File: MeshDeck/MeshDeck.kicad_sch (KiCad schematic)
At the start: 18 parts, among them CN1 ATGM336H-6N-74, SW1 4*4*1.7, SW2 4*4*1.7, U1 ESP32-S3-WROOM-1(N16R8), U2 SX1262S8S+T-X1, U5 RN32768114

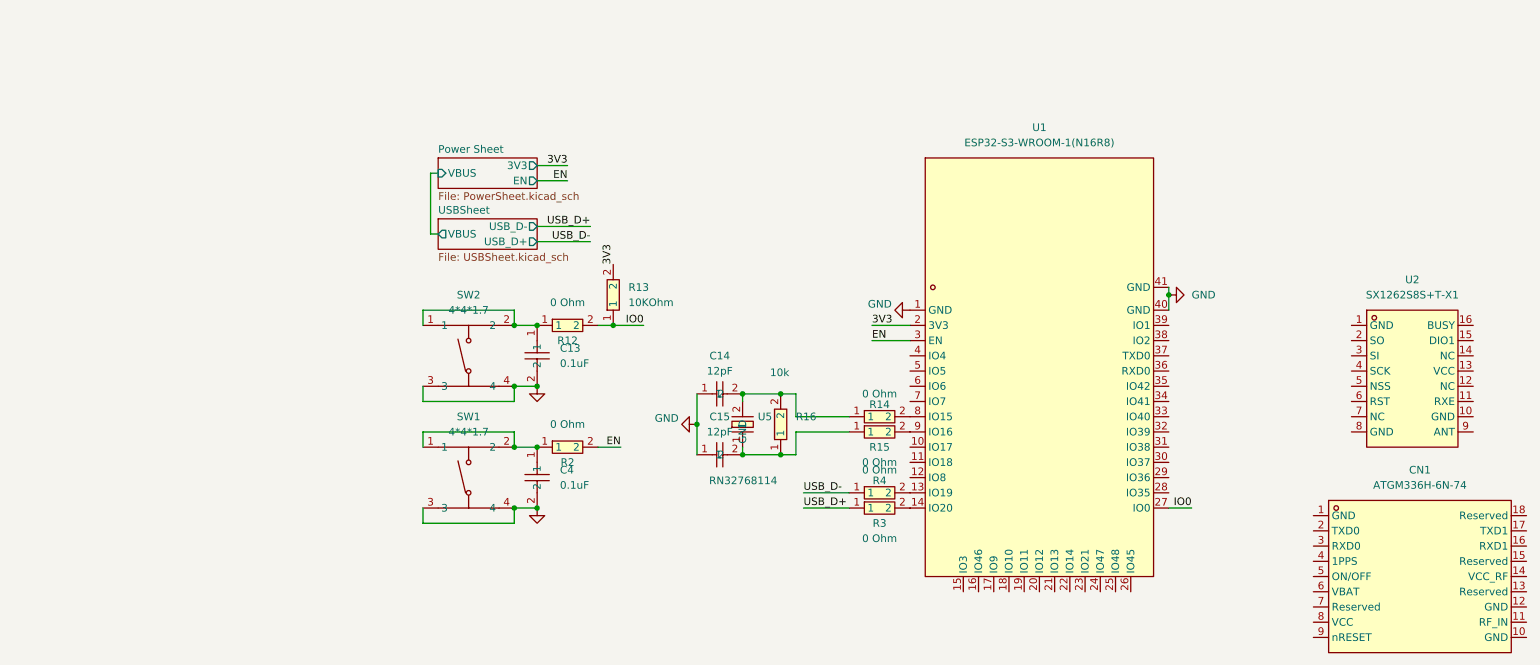
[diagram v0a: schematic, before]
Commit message: set up LoRa module and screen (wip)
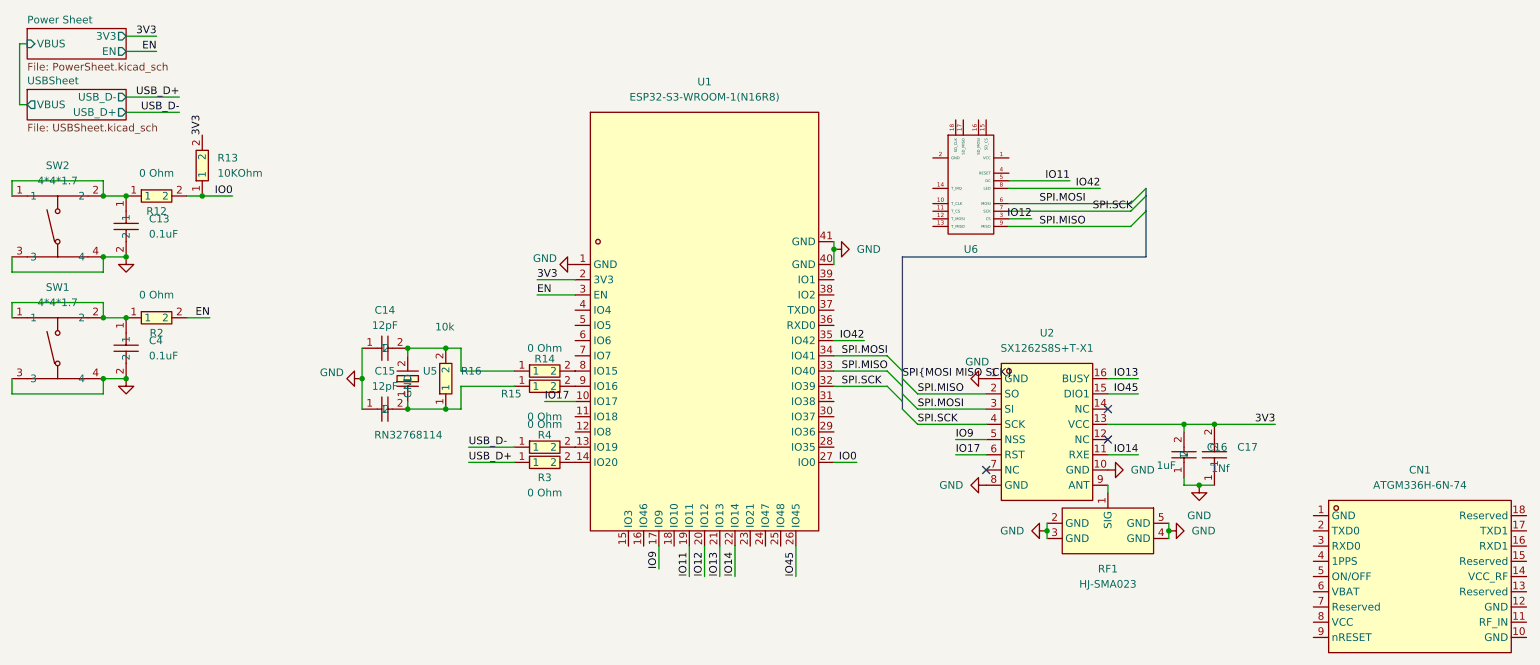
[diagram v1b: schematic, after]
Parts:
- added C16: 1uF, MeshDeck:C0402, symbol MeshDeck:CL05A105KP5NNNC
- added C17: 1Nf, MeshDeck:C0402, symbol MeshDeck:0402B102K500NT
- added RF1: HJ-SMA023, MeshDeck:SMA-SMD_HJ-SMA023, symbol MeshDeck:HJ-SMA023
- added U6: ~, MeshDeck:2.8 SPI LCD TFT ST7789, symbol MeshDeck:2.8_TFT_Touch_Screen
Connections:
- net 3V3: now also U2.13 (VCC), C16.2, C17.2
- net GND: now also U2.1 (GND), U2.10 (GND), U2.8 (GND), C16.1, C17.1, RF1.2 (GND), RF1.3 (GND), RF1.4 (GND), RF1.5 (GND)
- net IO14: now reaches U2.11 (RXE)
- net IO14: now also U1.22 (IO14)
- net IO45: now reaches U2.15 (DIO1)
- net IO45: now also U1.26 (IO45)
- net IO13: now reaches U2.16 (BUSY)
- net IO13: now also U1.21 (IO13)
- net SPI.MISO: now reaches U2.2 (SO)
- net SPI.MISO: now also U1.33 (IO40), U6.9 (MISO)
- net SPI.MOSI: now reaches U2.3 (SI)
- net SPI.MOSI: now also U1.34 (IO41), U6.6 (MOSI)
- net SPI.SCK: now reaches U2.4 (SCK)
- net SPI.SCK: now also U1.32 (IO39), U6.7 (SCK)
- net IO9: now reaches U2.5 (NSS)
- net IO9: now also U1.17 (IO9)
- net IO17: now reaches U2.6 (RST)
- net IO17: now also U1.10 (IO17)
- net at U2.9 (ANT): now also RF1.1 (SIG)
- net IO11: now reaches U1.19 (IO11)
- net IO11: now also U6.5 (DC)
- net IO12: now reaches U1.20 (IO12)
- net IO12: now also U6.3 (CS)
- net IO42: now reaches U1.35 (IO42)
- net IO42: now also U6.8 (LED)
- no-connect marks 0 -> 3
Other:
- moved on the sheet: C13, C14, C15, C4, R12, R13, R14, R15, R16, R2, R3, R4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
